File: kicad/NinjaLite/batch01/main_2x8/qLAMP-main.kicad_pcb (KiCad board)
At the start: 2 copper layers, 223.1 x 116 mm, 147 parts, among them J1 ALI_USB, J12 Conn_01x06_Male, J13 Conn_01x01_Male, J14 Conn_01x01_Male, J15 Conn_01x01_Male, J16 Conn_01x01_Male, J2 Barrel_Jack_Switch, J20 Conn_01x01_Male, J21 Conn_01x05_Male, J22 Conn_01x02_Male, J23 Conn_01x01_Male, J24 Conn_01x02_Male, J25 Conn_01x02_Male, J26 Conn_01x02_Male, J27 Conn_01x02_Male, J28 Conn_01x09_Male, Q1 Q_NMOS_GSD, Q3 Q_NMOS_GSD, Q5 Q_NMOS_GSD, U1 ADA2200ARUZ, U10 TLC5929, U11 IP2721, U12 TPS63710DRRR, U13 MCP1755T-3302E_DC, U14 MCP1755T-3302E_OT, U15 CJT1117-3.3, U16 CJT1117-5.0, U17 LITE_LCD, U18 SN74LVC1GU04DCKR, U19 CD74HC4067M96, U2 ADS1219IPWR, U20 CD74HC4067M96, U3 COM1305-0.032768-EXT-T-TR, U4 LMP7717MF_NOPB, U5 ESP32-WROOM-32, U6 ESP32-WROOM-32U, U7 SN74LVC1GU04DCKR, U8 TS12A12511DCNR, U9 CD74HC4067M96

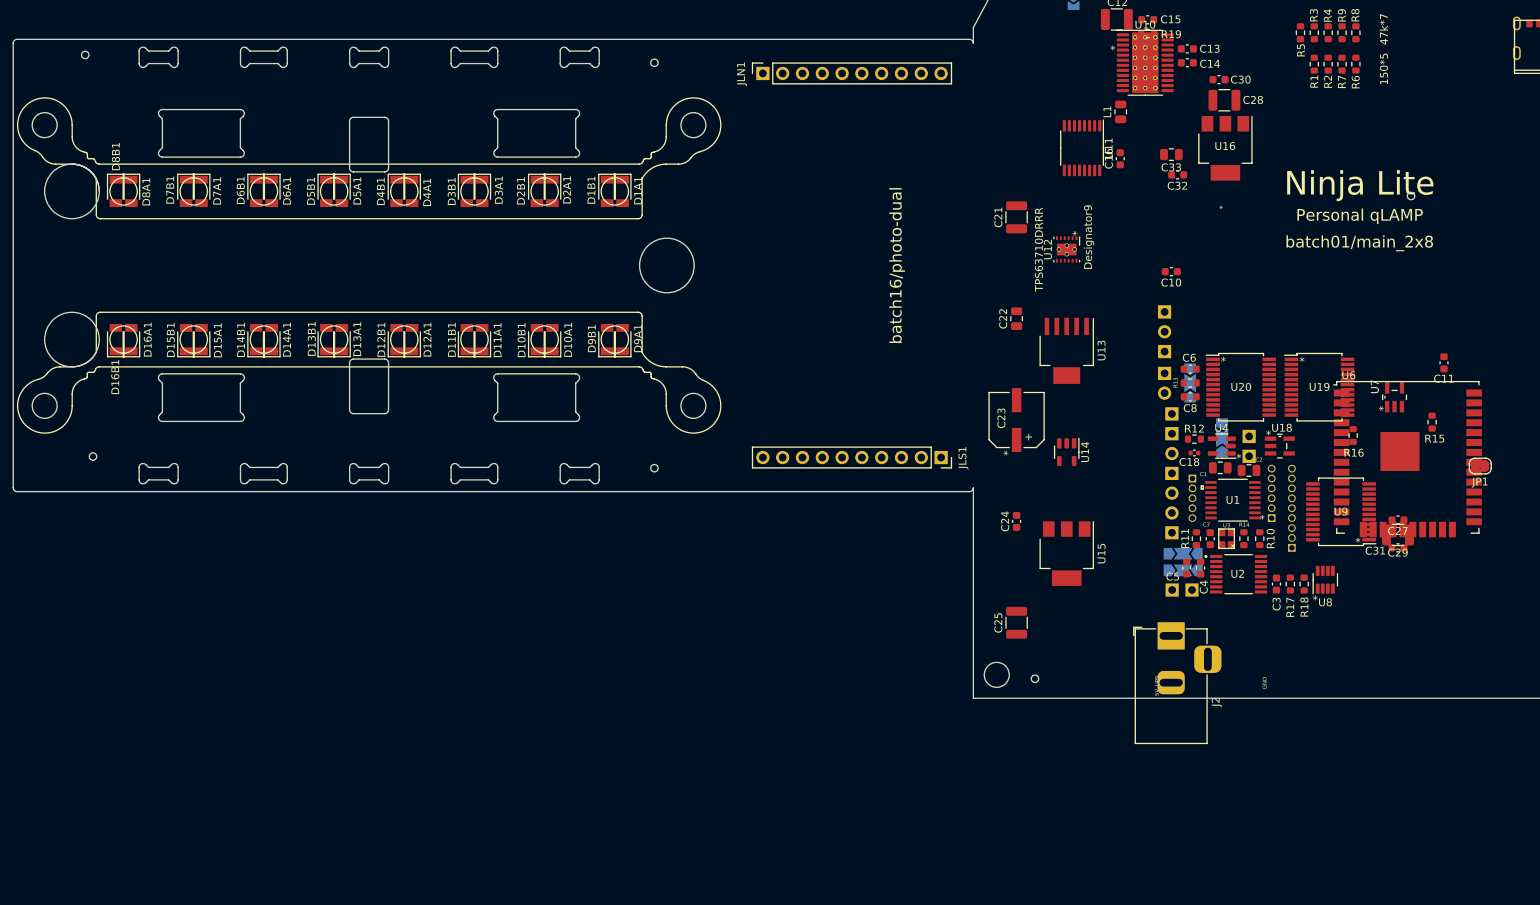
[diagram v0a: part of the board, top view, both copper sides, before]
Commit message: renmaed
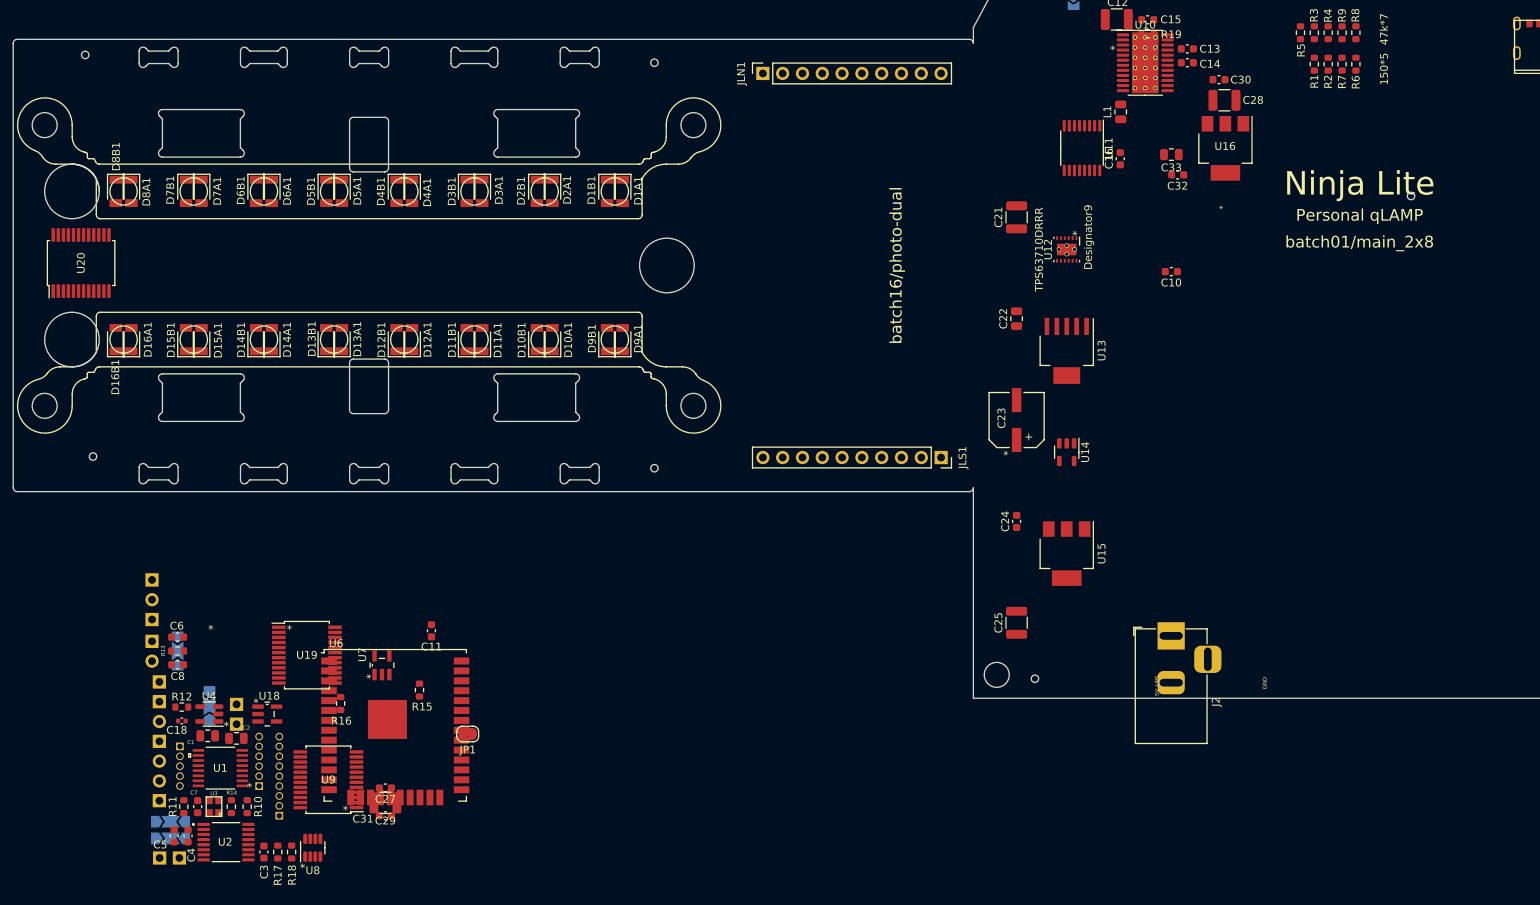
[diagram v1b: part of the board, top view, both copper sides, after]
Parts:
- moved U20 149.6 mm to (33.5, 94.7), turned to 90 degrees
- moved C27 134.3 mm to (72.5, 162.0)
- moved C5 134.3 mm to (45.4, 168.2)
- moved J15 134.3 mm to (46.1, 171.0)
- moved J16 134.3 mm to (43.5, 148.4)
- moved J22 134.3 mm to (43.5, 163.6)
- moved J26 134.3 mm to (43.5, 150.9)
- moved J27 134.3 mm to (43.5, 156.0)
- moved JP4 134.3 mm to (44.9, 166.3)
- moved JP5 134.3 mm to (44.9, 168.5)
- moved JP7 134.3 mm to (49.9, 151.5)
- moved R14 134.3 mm to (52.7, 164.4)
- moved R15 134.3 mm to (76.9, 149.5)
- moved R16 134.3 mm to (66.7, 151.2)
- moved U18 134.3 mm to (57.3, 152.5)
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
